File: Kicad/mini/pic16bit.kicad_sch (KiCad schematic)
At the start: 12 parts, among them K101 PE-450-4X6X-BLACK

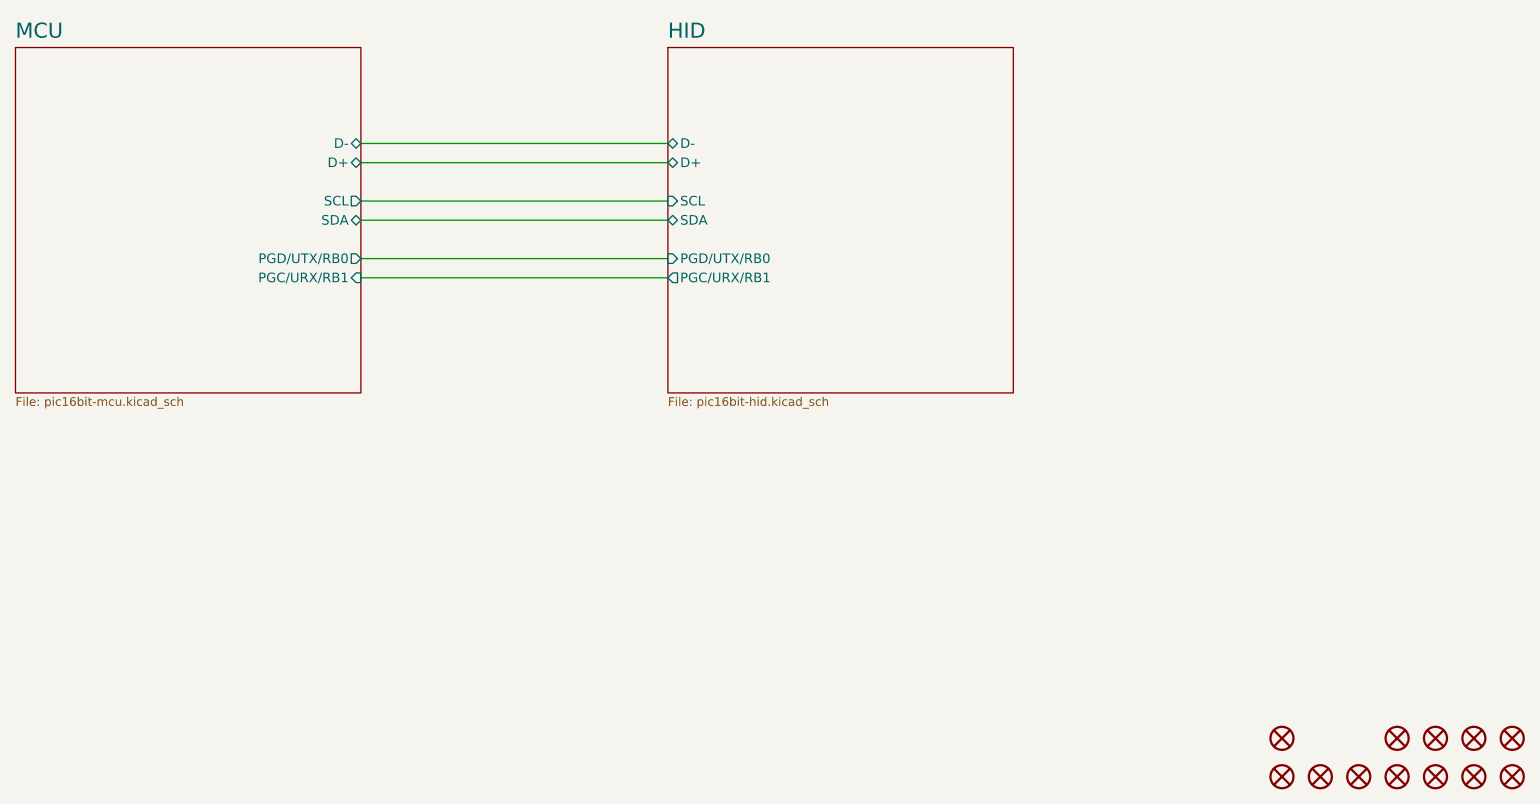
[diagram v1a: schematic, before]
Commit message: Update
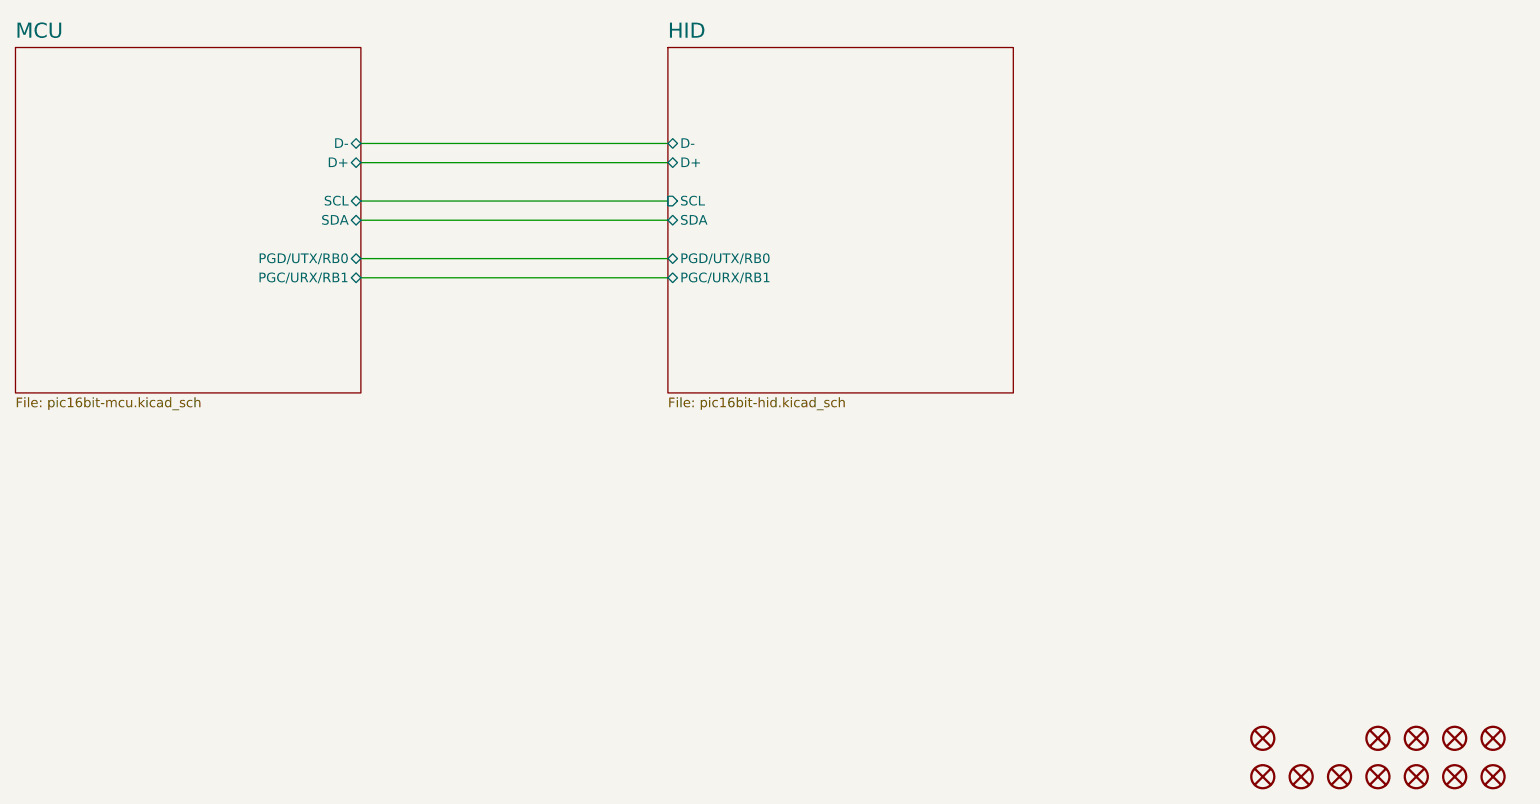
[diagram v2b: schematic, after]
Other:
- title: Diagram -> Connections
